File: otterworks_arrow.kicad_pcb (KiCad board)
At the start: 4 copper layers, 60 x 121 mm, 137 parts, among them U1 STM32F030C6Tx

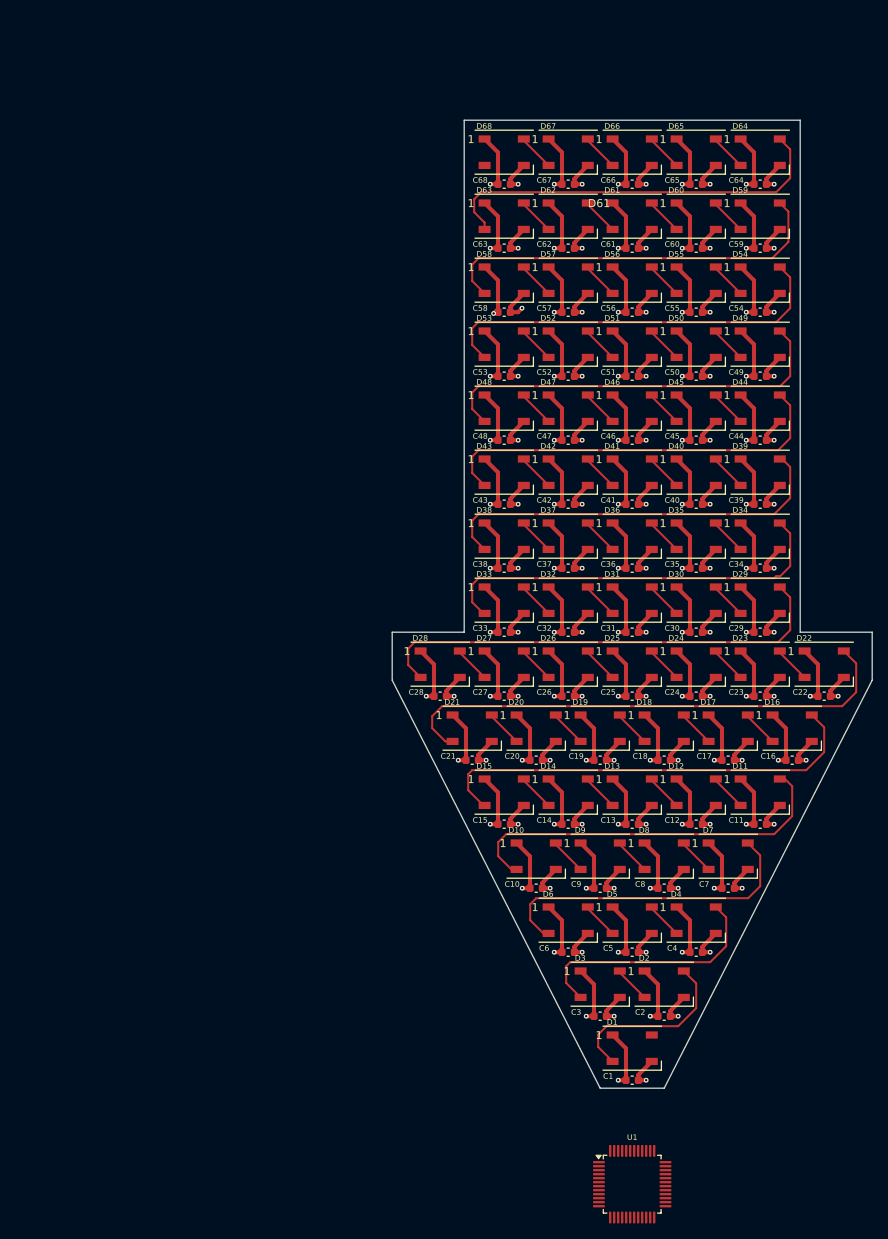
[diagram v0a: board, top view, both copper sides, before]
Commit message: bottom side done
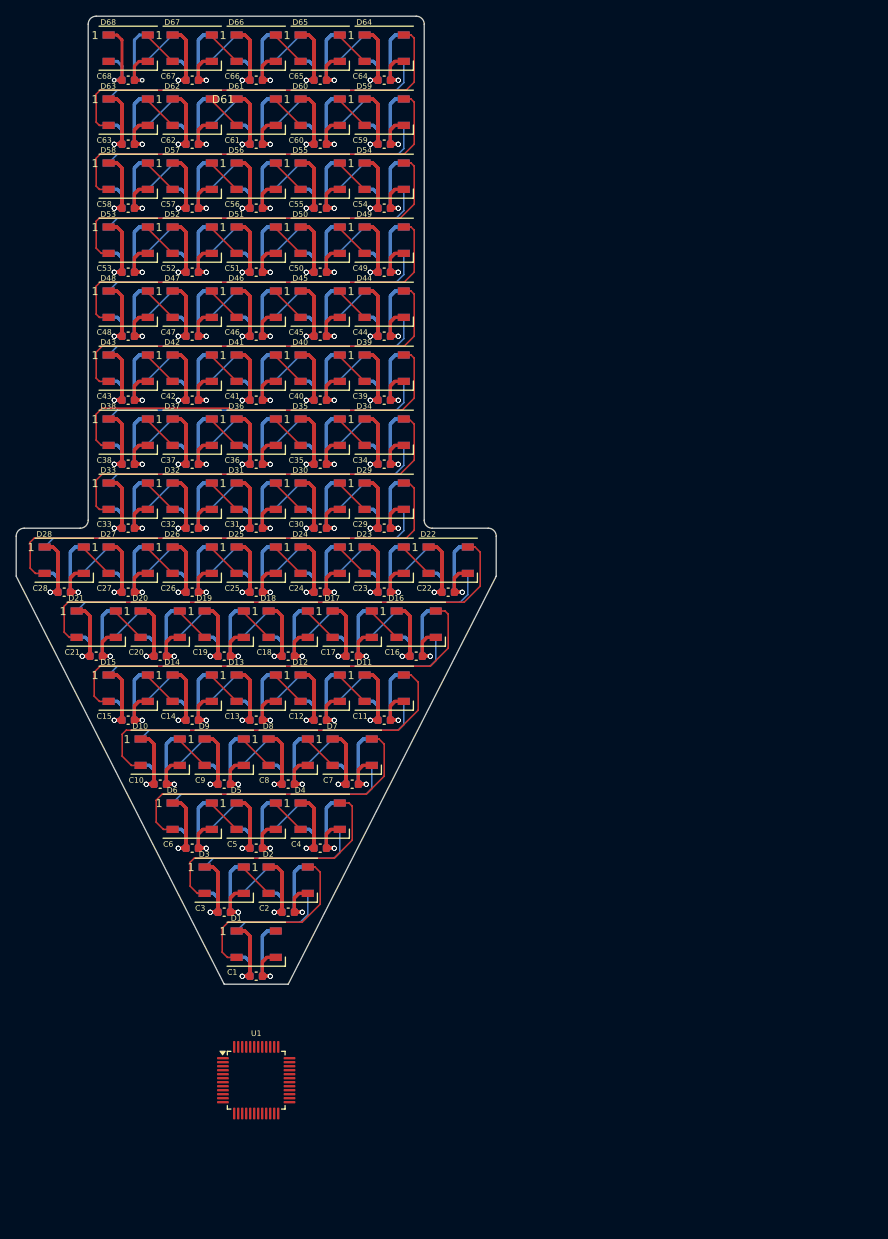
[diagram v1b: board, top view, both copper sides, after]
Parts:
- added C100: 100n, Capacitor_SMD:C_0603_1608Metric, B.Cu at (83.0, 125.0)
- added C101: 100n, Capacitor_SMD:C_0603_1608Metric, B.Cu at (75.0, 125.0)
- added C102: 100n, Capacitor_SMD:C_0603_1608Metric, B.Cu at (79.0, 133.0)
- added C103: 100n, Capacitor_SMD:C_0603_1608Metric, B.Cu at (83.0, 141.0)
- added C104: 100n, Capacitor_SMD:C_0603_1608Metric, B.Cu at (71.0, 101.0)
- added C105: 100n, Capacitor_SMD:C_0603_1608Metric, B.Cu at (87.0, 133.0)
- added C106: 100n, Capacitor_SMD:C_0603_1608Metric, B.Cu at (99.0, 53.0)
- added C107: 100n, Capacitor_SMD:C_0603_1608Metric, B.Cu at (75.0, 85.0)
- added C108: 100n, Capacitor_SMD:C_0603_1608Metric, B.Cu at (83.0, 109.0)
- added C109: 100n, Capacitor_SMD:C_0603_1608Metric, B.Cu at (83.0, 85.0)
- added C110: 100n, Capacitor_SMD:C_0603_1608Metric, B.Cu at (91.0, 53.0)
- added C111: 100n, Capacitor_SMD:C_0603_1608Metric, B.Cu at (91.0, 109.0)
- added C112: 100n, Capacitor_SMD:C_0603_1608Metric, B.Cu at (99.0, 109.0)
- added C113: 100n, Capacitor_SMD:C_0603_1608Metric, B.Cu at (75.0, 53.0)
- added C114: 100n, Capacitor_SMD:C_0603_1608Metric, B.Cu at (99.0, 45.0)
- added C115: 100n, Capacitor_SMD:C_0603_1608Metric, B.Cu at (67.0, 53.0)
- added C116: 100n, Capacitor_SMD:C_0603_1608Metric, B.Cu at (99.0, 61.0)
- added C117: 100n, Capacitor_SMD:C_0603_1608Metric, B.Cu at (59.0, 93.0)
- added C118: 100n, Capacitor_SMD:C_0603_1608Metric, B.Cu at (91.0, 85.0)
- added C119: 100n, Capacitor_SMD:C_0603_1608Metric, B.Cu at (91.0, 61.0)
- added C120: 100n, Capacitor_SMD:C_0603_1608Metric, B.Cu at (75.0, 61.0)
- added C121: 100n, Capacitor_SMD:C_0603_1608Metric, B.Cu at (99.0, 85.0)
- added C122: 100n, Capacitor_SMD:C_0603_1608Metric, B.Cu at (67.0, 109.0)
- added C123: 100n, Capacitor_SMD:C_0603_1608Metric, B.Cu at (87.0, 101.0)
- added C124: 100n, Capacitor_SMD:C_0603_1608Metric, B.Cu at (75.0, 109.0)
- added C125: 100n, Capacitor_SMD:C_0603_1608Metric, B.Cu at (103.0, 101.0)
- added C126: 100n, Capacitor_SMD:C_0603_1608Metric, B.Cu at (95.0, 101.0)
- added C127: 100n, Capacitor_SMD:C_0603_1608Metric, B.Cu at (83.0, 77.0)
- added C128: 100n, Capacitor_SMD:C_0603_1608Metric, B.Cu at (91.0, 77.0)
- added C129: 100n, Capacitor_SMD:C_0603_1608Metric, B.Cu at (99.0, 77.0)
- added C130: 100n, Capacitor_SMD:C_0603_1608Metric, B.Cu at (67.0, 85.0)
- added C131: 100n, Capacitor_SMD:C_0603_1608Metric, B.Cu at (83.0, 29.0)
- added C132: 100n, Capacitor_SMD:C_0603_1608Metric, B.Cu at (83.0, 53.0)
- added C133: 100n, Capacitor_SMD:C_0603_1608Metric, B.Cu at (67.0, 29.0)
- added C134: 100n, Capacitor_SMD:C_0603_1608Metric, B.Cu at (67.0, 61.0)
- added C135: 100n, Capacitor_SMD:C_0603_1608Metric, B.Cu at (75.0, 29.0)
- added C136: 100n, Capacitor_SMD:C_0603_1608Metric, B.Cu at (91.0, 29.0)
- added C69: 100n, Capacitor_SMD:C_0603_1608Metric, B.Cu at (79.0, 101.0)
- added C70: 100n, Capacitor_SMD:C_0603_1608Metric, B.Cu at (99.0, 69.0)
- added C71: 100n, Capacitor_SMD:C_0603_1608Metric, B.Cu at (75.0, 45.0)
- added C72: 100n, Capacitor_SMD:C_0603_1608Metric, B.Cu at (83.0, 45.0)
- added C73: 100n, Capacitor_SMD:C_0603_1608Metric, B.Cu at (67.0, 77.0)
- added C74: 100n, Capacitor_SMD:C_0603_1608Metric, B.Cu at (91.0, 45.0)
- added C75: 100n, Capacitor_SMD:C_0603_1608Metric, B.Cu at (75.0, 77.0)
- added C76: 100n, Capacitor_SMD:C_0603_1608Metric, B.Cu at (107.0, 93.0)
- added C77: 100n, Capacitor_SMD:C_0603_1608Metric, B.Cu at (83.0, 93.0)
- added C78: 100n, Capacitor_SMD:C_0603_1608Metric, B.Cu at (63.0, 101.0)
- added C79: 100n, Capacitor_SMD:C_0603_1608Metric, B.Cu at (99.0, 93.0)
- added C80: 100n, Capacitor_SMD:C_0603_1608Metric, B.Cu at (91.0, 93.0)
- added C81: 100n, Capacitor_SMD:C_0603_1608Metric, B.Cu at (91.0, 37.0)
- added C82: 100n, Capacitor_SMD:C_0603_1608Metric, B.Cu at (75.0, 37.0)
- added C83: 100n, Capacitor_SMD:C_0603_1608Metric, B.Cu at (67.0, 37.0)
- added C84: 100n, Capacitor_SMD:C_0603_1608Metric, B.Cu at (83.0, 37.0)
- added C85: 100n, Capacitor_SMD:C_0603_1608Metric, B.Cu at (83.0, 61.0)
- added C86: 100n, Capacitor_SMD:C_0603_1608Metric, B.Cu at (99.0, 29.0)
- added C87: 100n, Capacitor_SMD:C_0603_1608Metric, B.Cu at (67.0, 69.0)
- added C88: 100n, Capacitor_SMD:C_0603_1608Metric, B.Cu at (95.0, 117.0)
- added C89: 100n, Capacitor_SMD:C_0603_1608Metric, B.Cu at (87.0, 117.0)
- added C90: 100n, Capacitor_SMD:C_0603_1608Metric, B.Cu at (79.0, 117.0)
- added C91: 100n, Capacitor_SMD:C_0603_1608Metric, B.Cu at (71.0, 117.0)
- added C92: 100n, Capacitor_SMD:C_0603_1608Metric, B.Cu at (67.0, 93.0)
- added C93: 100n, Capacitor_SMD:C_0603_1608Metric, B.Cu at (75.0, 93.0)
- added C94: 100n, Capacitor_SMD:C_0603_1608Metric, B.Cu at (83.0, 69.0)
- added C95: 100n, Capacitor_SMD:C_0603_1608Metric, B.Cu at (67.0, 45.0)
- added C96: 100n, Capacitor_SMD:C_0603_1608Metric, B.Cu at (75.0, 69.0)
- added C97: 100n, Capacitor_SMD:C_0603_1608Metric, B.Cu at (99.0, 37.0)
- added C98: 100n, Capacitor_SMD:C_0603_1608Metric, B.Cu at (91.0, 69.0)
- added C99: 100n, Capacitor_SMD:C_0603_1608Metric, B.Cu at (91.0, 125.0)
- added D100: WS2812B-2020, LED_SMD:LED_WS2812B_PLCC4_5.0x5.0mm_P3.2mm, B.Cu at (83.0, 121.0)
- added D101: WS2812B-2020, LED_SMD:LED_WS2812B_PLCC4_5.0x5.0mm_P3.2mm, B.Cu at (75.0, 121.0)
- added D102: WS2812B-2020, LED_SMD:LED_WS2812B_PLCC4_5.0x5.0mm_P3.2mm, B.Cu at (79.0, 129.0)
- added D103: WS2812B-2020, LED_SMD:LED_WS2812B_PLCC4_5.0x5.0mm_P3.2mm, B.Cu at (83.0, 137.0)
- added D104: WS2812B-2020, LED_SMD:LED_WS2812B_PLCC4_5.0x5.0mm_P3.2mm, B.Cu at (71.0, 97.0)
- added D105: WS2812B-2020, LED_SMD:LED_WS2812B_PLCC4_5.0x5.0mm_P3.2mm, B.Cu at (87.0, 129.0)
- added D106: WS2812B-2020, LED_SMD:LED_WS2812B_PLCC4_5.0x5.0mm_P3.2mm, B.Cu at (99.0, 49.0)
- added D107: WS2812B-2020, LED_SMD:LED_WS2812B_PLCC4_5.0x5.0mm_P3.2mm, B.Cu at (75.0, 81.0)
- added D108: WS2812B-2020, LED_SMD:LED_WS2812B_PLCC4_5.0x5.0mm_P3.2mm, B.Cu at (83.0, 105.0)
- added D109: WS2812B-2020, LED_SMD:LED_WS2812B_PLCC4_5.0x5.0mm_P3.2mm, B.Cu at (83.0, 81.0)
- added D110: WS2812B-2020, LED_SMD:LED_WS2812B_PLCC4_5.0x5.0mm_P3.2mm, B.Cu at (91.0, 49.0)
- added D111: WS2812B-2020, LED_SMD:LED_WS2812B_PLCC4_5.0x5.0mm_P3.2mm, B.Cu at (91.0, 105.0)
- added D112: WS2812B-2020, LED_SMD:LED_WS2812B_PLCC4_5.0x5.0mm_P3.2mm, B.Cu at (99.0, 105.0)
- added D113: WS2812B-2020, LED_SMD:LED_WS2812B_PLCC4_5.0x5.0mm_P3.2mm, B.Cu at (75.0, 49.0)
- added D114: WS2812B-2020, LED_SMD:LED_WS2812B_PLCC4_5.0x5.0mm_P3.2mm, B.Cu at (99.0, 41.0)
- added D115: WS2812B-2020, LED_SMD:LED_WS2812B_PLCC4_5.0x5.0mm_P3.2mm, B.Cu at (67.0, 49.0)
- added D116: WS2812B-2020, LED_SMD:LED_WS2812B_PLCC4_5.0x5.0mm_P3.2mm, B.Cu at (99.0, 57.0)
- added D117: WS2812B-2020, LED_SMD:LED_WS2812B_PLCC4_5.0x5.0mm_P3.2mm, B.Cu at (59.0, 89.0)
- added D118: WS2812B-2020, LED_SMD:LED_WS2812B_PLCC4_5.0x5.0mm_P3.2mm, B.Cu at (91.0, 81.0)
- added D119: WS2812B-2020, LED_SMD:LED_WS2812B_PLCC4_5.0x5.0mm_P3.2mm, B.Cu at (91.0, 57.0)
- added D120: WS2812B-2020, LED_SMD:LED_WS2812B_PLCC4_5.0x5.0mm_P3.2mm, B.Cu at (75.0, 57.0)
- added D121: WS2812B-2020, LED_SMD:LED_WS2812B_PLCC4_5.0x5.0mm_P3.2mm, B.Cu at (99.0, 81.0)
- added D122: WS2812B-2020, LED_SMD:LED_WS2812B_PLCC4_5.0x5.0mm_P3.2mm, B.Cu at (67.0, 105.0)
- added D123: WS2812B-2020, LED_SMD:LED_WS2812B_PLCC4_5.0x5.0mm_P3.2mm, B.Cu at (87.0, 97.0)
- added D124: WS2812B-2020, LED_SMD:LED_WS2812B_PLCC4_5.0x5.0mm_P3.2mm, B.Cu at (75.0, 105.0)
- added D125: WS2812B-2020, LED_SMD:LED_WS2812B_PLCC4_5.0x5.0mm_P3.2mm, B.Cu at (103.0, 97.0)
- added D126: WS2812B-2020, LED_SMD:LED_WS2812B_PLCC4_5.0x5.0mm_P3.2mm, B.Cu at (95.0, 97.0)
- added D127: WS2812B-2020, LED_SMD:LED_WS2812B_PLCC4_5.0x5.0mm_P3.2mm, B.Cu at (83.0, 73.0)
- added D128: WS2812B-2020, LED_SMD:LED_WS2812B_PLCC4_5.0x5.0mm_P3.2mm, B.Cu at (91.0, 73.0)
- added D129: WS2812B-2020, LED_SMD:LED_WS2812B_PLCC4_5.0x5.0mm_P3.2mm, B.Cu at (99.0, 73.0)
- added D130: WS2812B-2020, LED_SMD:LED_WS2812B_PLCC4_5.0x5.0mm_P3.2mm, B.Cu at (67.0, 81.0)
- added D131: WS2812B-2020, LED_SMD:LED_WS2812B_PLCC4_5.0x5.0mm_P3.2mm, B.Cu at (83.0, 25.0)
- added D132: WS2812B-2020, LED_SMD:LED_WS2812B_PLCC4_5.0x5.0mm_P3.2mm, B.Cu at (83.0, 49.0)
- added D133: WS2812B-2020, LED_SMD:LED_WS2812B_PLCC4_5.0x5.0mm_P3.2mm, B.Cu at (67.0, 25.0)
- added D134: WS2812B-2020, LED_SMD:LED_WS2812B_PLCC4_5.0x5.0mm_P3.2mm, B.Cu at (67.0, 57.0)
- added D135: WS2812B-2020, LED_SMD:LED_WS2812B_PLCC4_5.0x5.0mm_P3.2mm, B.Cu at (75.0, 25.0)
- added D136: WS2812B-2020, LED_SMD:LED_WS2812B_PLCC4_5.0x5.0mm_P3.2mm, B.Cu at (91.0, 25.0)
- added D69: WS2812B-2020, LED_SMD:LED_WS2812B_PLCC4_5.0x5.0mm_P3.2mm, B.Cu at (79.0, 97.0)
- added D70: WS2812B-2020, LED_SMD:LED_WS2812B_PLCC4_5.0x5.0mm_P3.2mm, B.Cu at (99.0, 65.0)
- added D71: WS2812B-2020, LED_SMD:LED_WS2812B_PLCC4_5.0x5.0mm_P3.2mm, B.Cu at (75.0, 41.0)
- added D72: WS2812B-2020, LED_SMD:LED_WS2812B_PLCC4_5.0x5.0mm_P3.2mm, B.Cu at (83.0, 41.0)
- added D73: WS2812B-2020, LED_SMD:LED_WS2812B_PLCC4_5.0x5.0mm_P3.2mm, B.Cu at (67.0, 73.0)
- added D74: WS2812B-2020, LED_SMD:LED_WS2812B_PLCC4_5.0x5.0mm_P3.2mm, B.Cu at (91.0, 41.0)
- added D75: WS2812B-2020, LED_SMD:LED_WS2812B_PLCC4_5.0x5.0mm_P3.2mm, B.Cu at (75.0, 73.0)
- added D76: WS2812B-2020, LED_SMD:LED_WS2812B_PLCC4_5.0x5.0mm_P3.2mm, B.Cu at (107.0, 89.0)
- added D77: WS2812B-2020, LED_SMD:LED_WS2812B_PLCC4_5.0x5.0mm_P3.2mm, B.Cu at (83.0, 89.0)
- added D78: WS2812B-2020, LED_SMD:LED_WS2812B_PLCC4_5.0x5.0mm_P3.2mm, B.Cu at (63.0, 97.0)
- added D79: WS2812B-2020, LED_SMD:LED_WS2812B_PLCC4_5.0x5.0mm_P3.2mm, B.Cu at (99.0, 89.0)
- added D80: WS2812B-2020, LED_SMD:LED_WS2812B_PLCC4_5.0x5.0mm_P3.2mm, B.Cu at (91.0, 89.0)
- added D81: WS2812B-2020, LED_SMD:LED_WS2812B_PLCC4_5.0x5.0mm_P3.2mm, B.Cu at (91.0, 33.0)
- added D82: WS2812B-2020, LED_SMD:LED_WS2812B_PLCC4_5.0x5.0mm_P3.2mm, B.Cu at (75.0, 33.0)
- added D83: WS2812B-2020, LED_SMD:LED_WS2812B_PLCC4_5.0x5.0mm_P3.2mm, B.Cu at (67.0, 33.0)
- added D84: WS2812B-2020, LED_SMD:LED_WS2812B_PLCC4_5.0x5.0mm_P3.2mm, B.Cu at (83.0, 33.0)
- added D85: WS2812B-2020, LED_SMD:LED_WS2812B_PLCC4_5.0x5.0mm_P3.2mm, B.Cu at (83.0, 57.0)
- added D86: WS2812B-2020, LED_SMD:LED_WS2812B_PLCC4_5.0x5.0mm_P3.2mm, B.Cu at (99.0, 25.0)
- added D87: WS2812B-2020, LED_SMD:LED_WS2812B_PLCC4_5.0x5.0mm_P3.2mm, B.Cu at (67.0, 65.0)
- added D88: WS2812B-2020, LED_SMD:LED_WS2812B_PLCC4_5.0x5.0mm_P3.2mm, B.Cu at (95.0, 113.0)
- added D89: WS2812B-2020, LED_SMD:LED_WS2812B_PLCC4_5.0x5.0mm_P3.2mm, B.Cu at (87.0, 113.0)
- added D90: WS2812B-2020, LED_SMD:LED_WS2812B_PLCC4_5.0x5.0mm_P3.2mm, B.Cu at (79.0, 113.0)
- added D91: WS2812B-2020, LED_SMD:LED_WS2812B_PLCC4_5.0x5.0mm_P3.2mm, B.Cu at (71.0, 113.0)
- added D92: WS2812B-2020, LED_SMD:LED_WS2812B_PLCC4_5.0x5.0mm_P3.2mm, B.Cu at (67.0, 89.0)
- added D93: WS2812B-2020, LED_SMD:LED_WS2812B_PLCC4_5.0x5.0mm_P3.2mm, B.Cu at (75.0, 89.0)
- added D94: WS2812B-2020, LED_SMD:LED_WS2812B_PLCC4_5.0x5.0mm_P3.2mm, B.Cu at (83.0, 65.0)
- added D95: WS2812B-2020, LED_SMD:LED_WS2812B_PLCC4_5.0x5.0mm_P3.2mm, B.Cu at (67.0, 41.0)
- added D96: WS2812B-2020, LED_SMD:LED_WS2812B_PLCC4_5.0x5.0mm_P3.2mm, B.Cu at (75.0, 65.0)
- added D97: WS2812B-2020, LED_SMD:LED_WS2812B_PLCC4_5.0x5.0mm_P3.2mm, B.Cu at (99.0, 33.0)
- added D98: WS2812B-2020, LED_SMD:LED_WS2812B_PLCC4_5.0x5.0mm_P3.2mm, B.Cu at (91.0, 65.0)
- added D99: WS2812B-2020, LED_SMD:LED_WS2812B_PLCC4_5.0x5.0mm_P3.2mm, B.Cu at (91.0, 121.0)
- moved C1 48.8 mm to (83.0, 141.0)
- moved C10 48.8 mm to (71.0, 117.0)
- moved C11 48.8 mm to (99.0, 109.0)
- moved C12 48.8 mm to (91.0, 109.0)
- moved C13 48.8 mm to (83.0, 109.0)
- moved C14 48.8 mm to (75.0, 109.0)
- moved C15 48.8 mm to (67.0, 109.0)
- moved C16 48.8 mm to (103.0, 101.0)
- moved C17 48.8 mm to (95.0, 101.0)
- moved C18 48.8 mm to (87.0, 101.0)
- moved C19 48.8 mm to (79.0, 101.0)
- moved C2 48.8 mm to (87.0, 133.0)
- moved C20 48.8 mm to (71.0, 101.0)
- moved C21 48.8 mm to (63.0, 101.0)
- moved C22 48.8 mm to (107.0, 93.0)
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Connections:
- U1 pad 29: unconnected-(U1-PA8-Pad29) -> /leds1/DIN
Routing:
- net GND: track 274.0 -> 3076.2 mm, vias 68 -> 269
- net +5V: track 497.3 -> 2857.0 mm, vias 68 -> 269
- net /leds1/ws2812_21/DOUT: track 0.00 -> 52.8 mm
- net /leds1/ws2812_28/DOUT: track 0.00 -> 48.8 mm
- net /leds1/ws2812_15/DOUT: track 0.00 -> 44.9 mm
- net /leds1/ws2812_58/DOUT: track 0.00 -> 40.9 mm
- net /leds1/ws2812_63/DOUT: track 0.00 -> 40.8 mm
- net /leds1/ws2812_48/DOUT: track 0.00 -> 40.8 mm
- net /leds1/ws2812_38/DOUT: track 0.00 -> 40.8 mm
- net /leds1/ws2812_53/DOUT: track 0.00 -> 40.8 mm
- net /leds1/ws2812_43/DOUT: track 0.00 -> 40.8 mm
- net /leds1/ws2812_33/DOUT: track 0.00 -> 40.7 mm
- net /leds1/ws2812_10/DOUT: track 0.00 -> 36.9 mm
- net /leds1/ws2812_6/DOUT: track 0.00 -> 28.9 mm
- net /leds1/ws2812_3/DOUT: track 0.00 -> 20.9 mm
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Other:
- outline, holes or cut-outs redrawn
